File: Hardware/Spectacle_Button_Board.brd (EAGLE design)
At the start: 44.5 x 73.7 mm, 46 parts, among them J17 AUDIO-JACK3, J19 FTDI_DEVICE, J20 AUDIO-JACK3, U1 CY8C4146LQI-S422, U2 3.3V/150mA

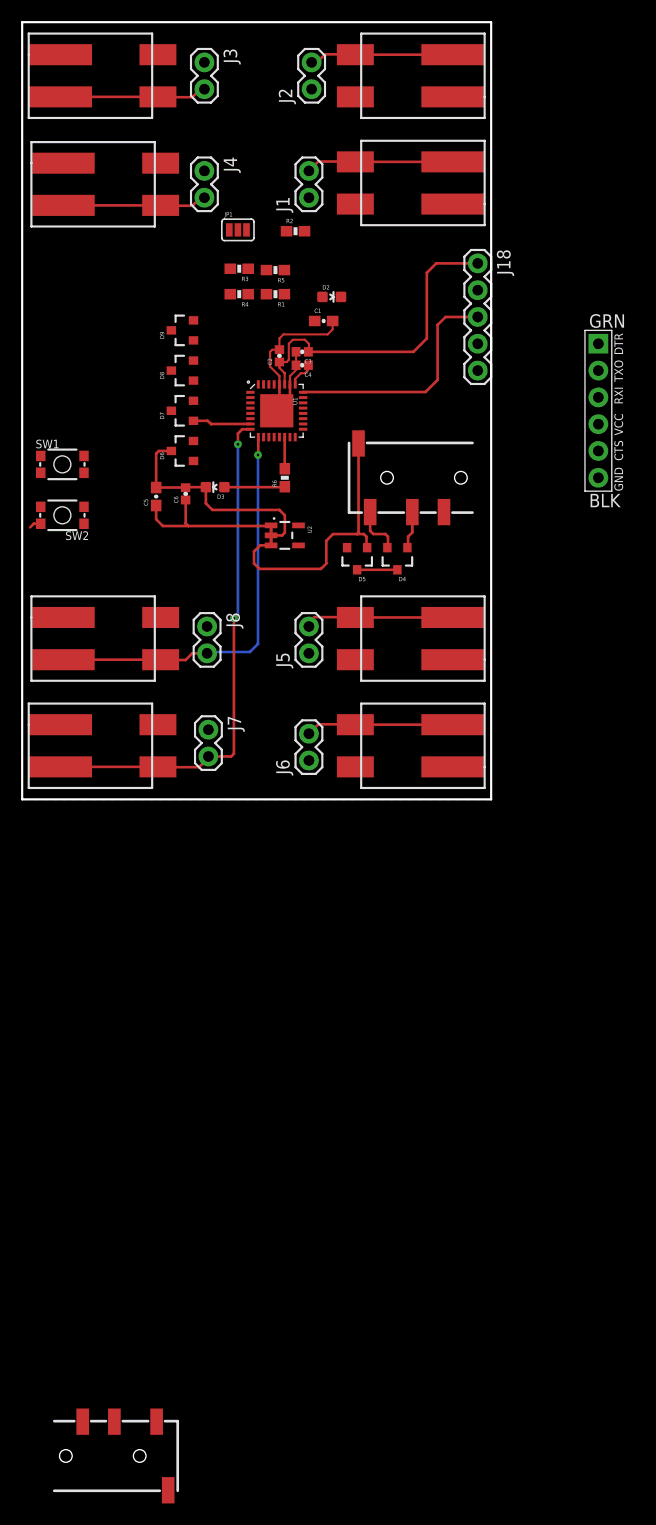
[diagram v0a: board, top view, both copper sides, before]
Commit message: partially routed
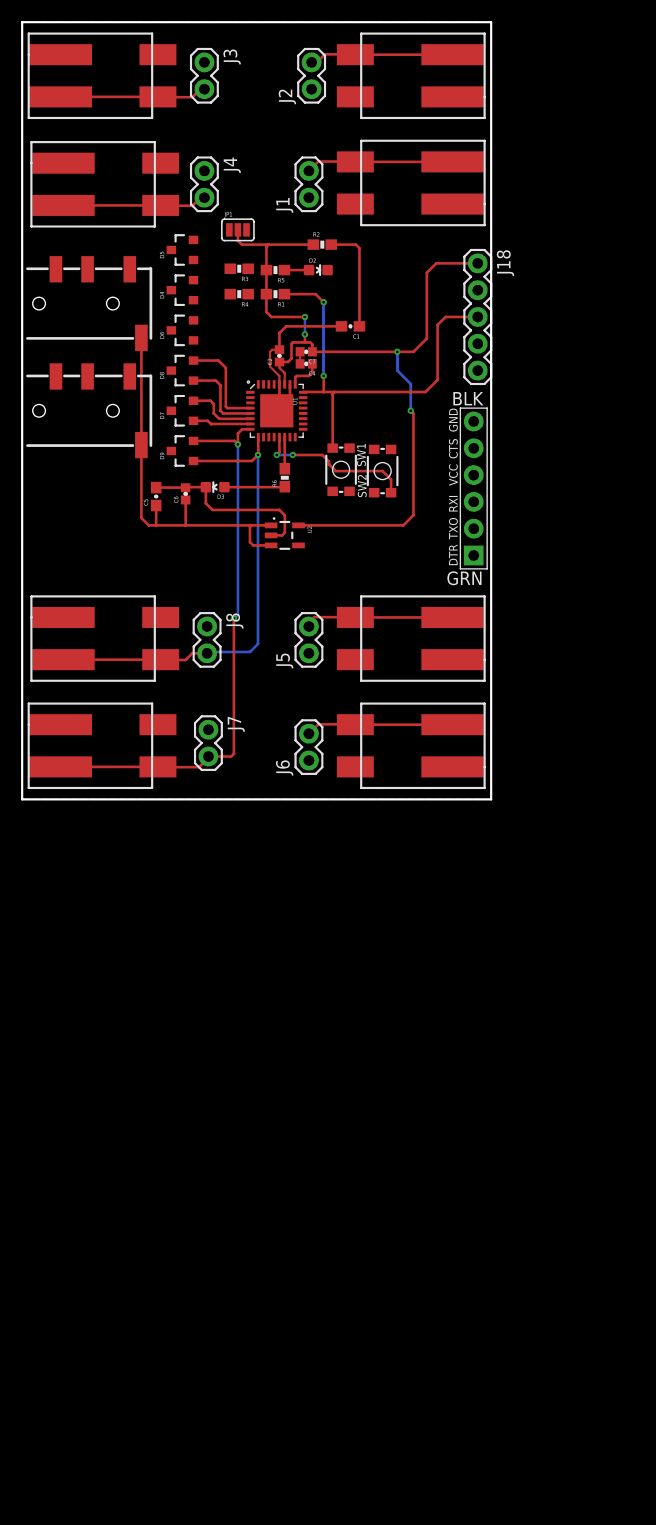
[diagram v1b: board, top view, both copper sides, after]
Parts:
- moved J20 109.2 mm to (-31.8, 38.1)
- moved J17 43.6 mm to (-31.8, 27.9), turned to 0 degrees
- moved D5 33.6 mm to (-16.5, 43.2), turned to 90 degrees
- moved D4 32.5 mm to (-16.5, 39.4), turned to 90 degrees
- moved SW2 30.6 mm to (2.41, 22.2), turned to 90 degrees
- moved SW1 26.4 mm to (-1.52, 22.4), turned to 270 degrees
- moved J19 13.9 mm to (11.0, 20.6), turned to 90 degrees
- moved D6 11.4 mm to (-16.5, 35.6)
- moved D9 11.4 mm to (-16.5, 24.1)
- moved D2 2.84 mm to (-3.68, 41.3)
- moved R2 2.84 mm to (-3.30, 43.7)
- moved C1 2.59 mm to (-0.64, 35.9), turned to 180 degrees
- moved C4 0.40 mm to (-4.83, 32.4)
- moved C3 0.38 mm to (-4.83, 33.5)
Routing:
- net 3.3V: track 31.0 -> 79.1 mm, vias 0 -> 4
- net XRES: track 22.6 -> 40.5 mm, vias 0 -> 2
- net BTN: track 0.00 -> 15.0 mm, vias 0 -> 2
- net GND: track 48.8 -> 37.4 mm
- net N$3: track 0.00 -> 10.2 mm
- net IN_2: track 14.0 -> 23.4 mm
- net IN_3: track 13.7 -> 21.8 mm
- net IN_4: track 14.3 -> 20.9 mm
- net IN_7: track 38.7 -> 45.1 mm
- net VIN: track 43.3 -> 37.7 mm
- net SDA: track 4.77 -> 0.00 mm
- net IN_6: track 48.9 -> 53.3 mm
- net SCL: track 3.56 -> 0.00 mm
- net N$4: track 0.00 -> 2.34 mm
- net VCC: track 2.56 -> 3.29 mm
